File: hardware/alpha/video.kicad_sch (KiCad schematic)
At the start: 104 parts, among them J1 BANK2_AUX, J2 OUT1, J3 OUT2, U1 L78L05_SO8, U3 L79L05_SO8, U4 AD768, U5 MAX4104, U6 AD8620, U7 MAX4104, U8 MCP47FEB22A0-E/ST

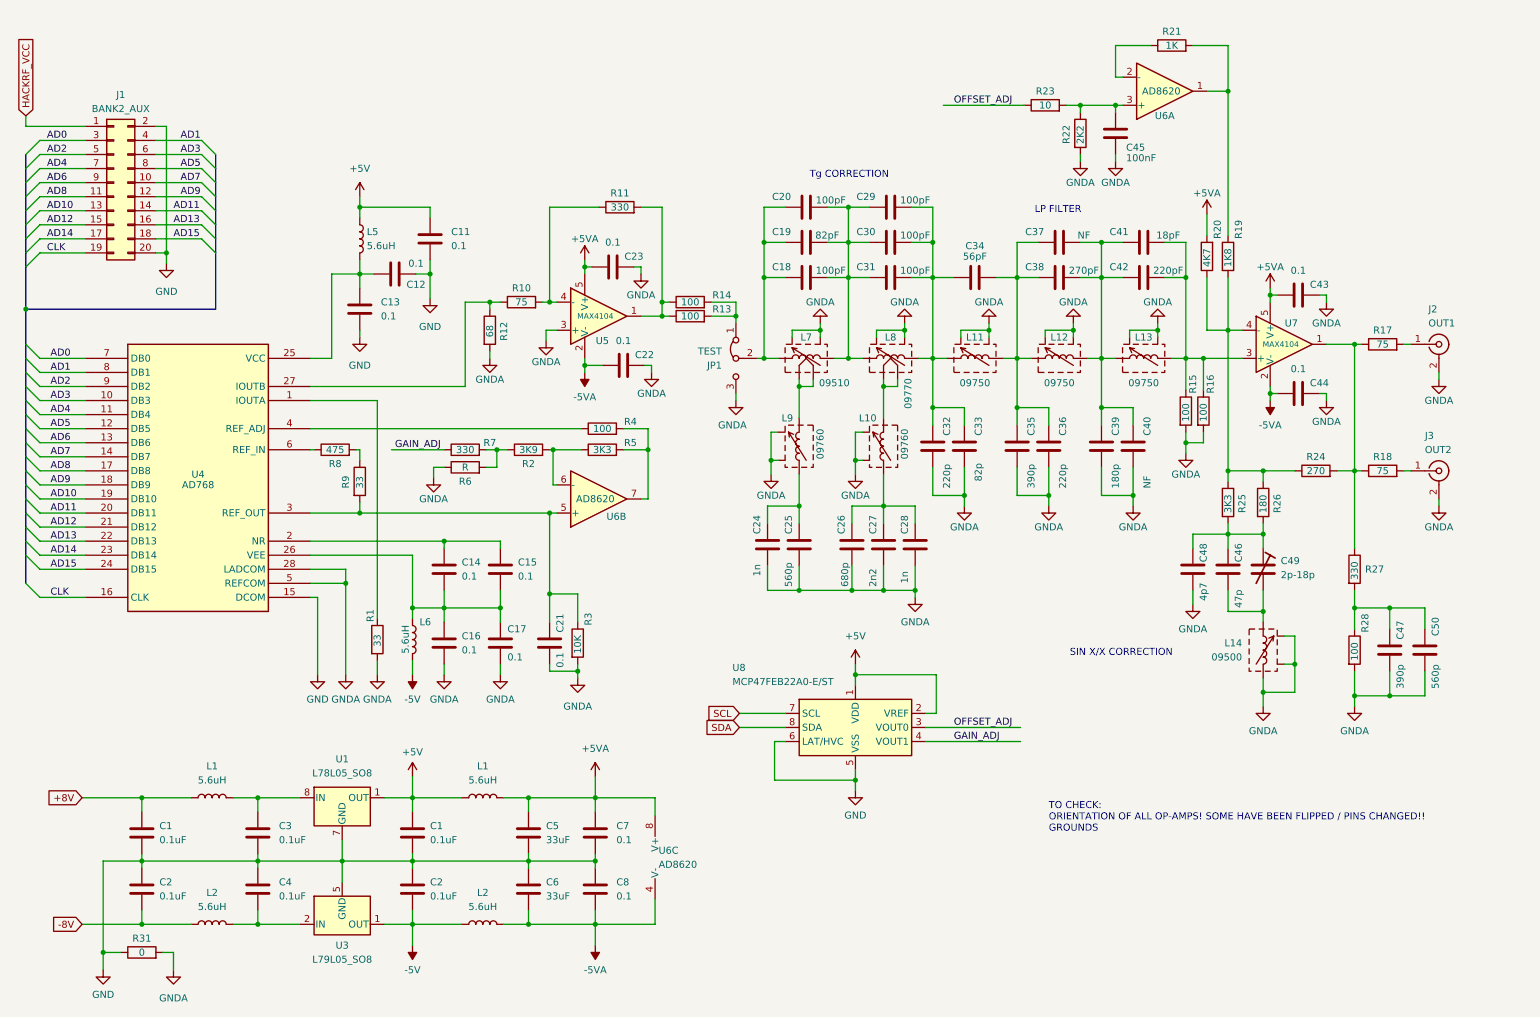
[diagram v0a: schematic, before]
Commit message: Updated
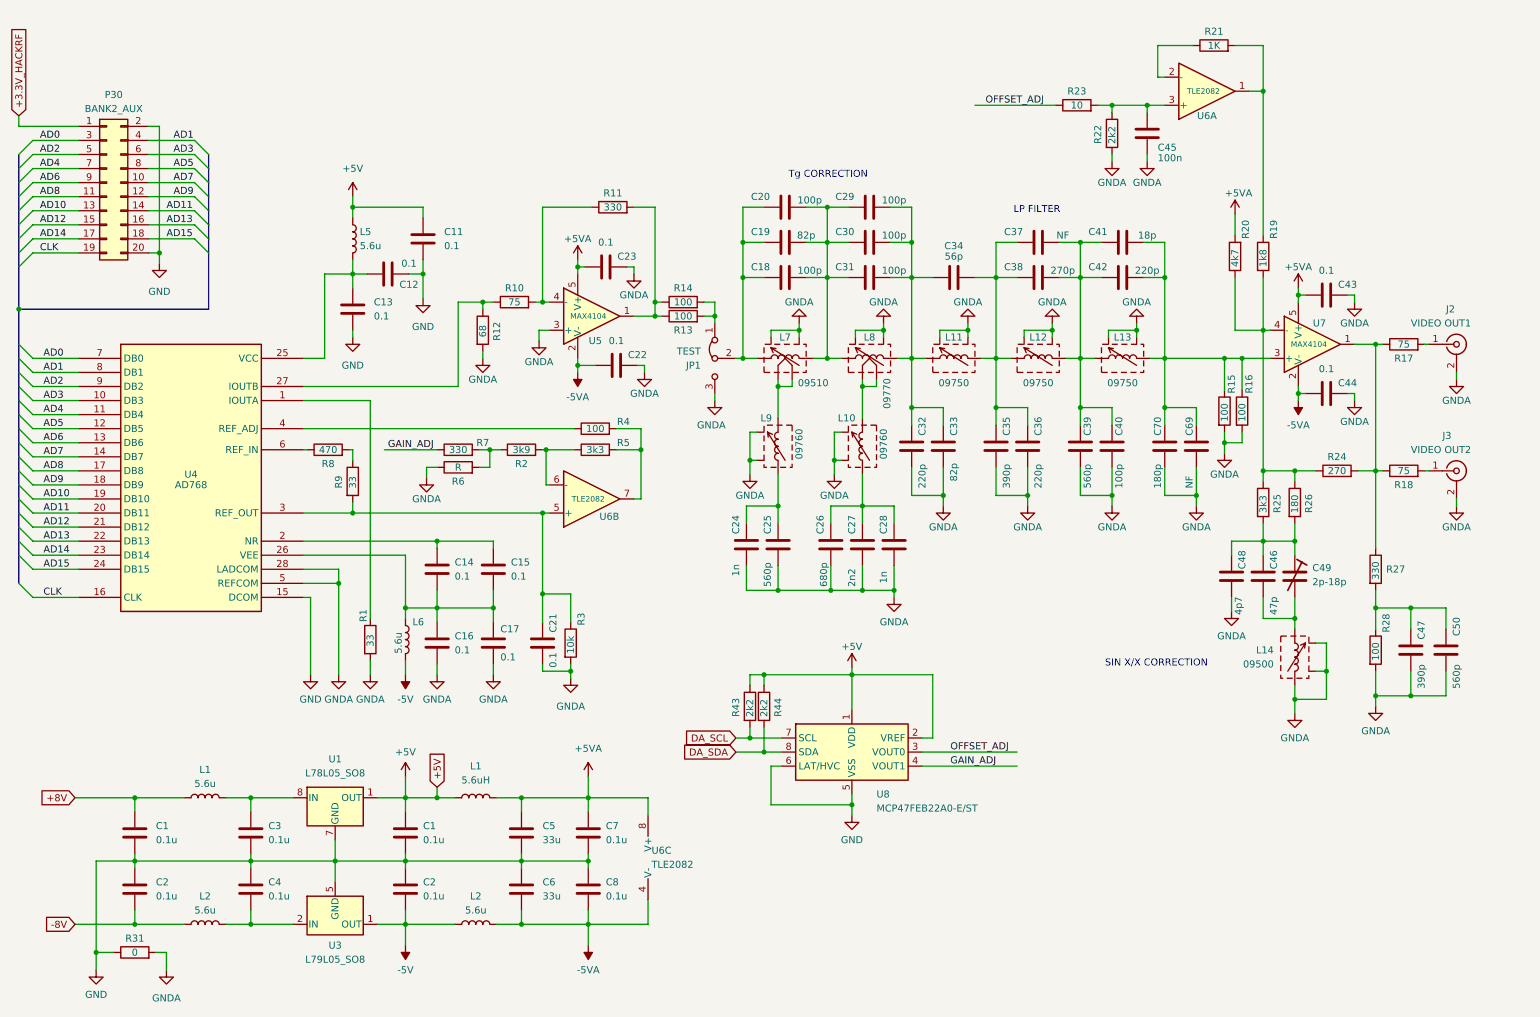
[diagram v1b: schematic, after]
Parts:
- added C69: NF, symbol Device:C
- added C70: 180p, symbol Device:C
- added R43, R44: 2k2, symbol Device:R
- C1, C2, C3, C4: value 0.1uF -> 0.1u
- C18, C20, C29, C30, C31: value 100pF -> 100p
- C19: value 82pF -> 82p
- C34: value 56pF -> 56p
- C38: value 270pF -> 270p
- C39: value 180p -> 560p
- C40: value NF -> 100p
- C41: value 18pF -> 18p
- C42: value 220pF -> 220p
- C45: value 100nF -> 100n
- C5, C6: value 33uF -> 33u
- C7, C8: value 0.1 -> 0.1u
- J2: value OUT1 -> VIDEO OUT1
- J3: value OUT2 -> VIDEO OUT2
- L1, L2, L5, L6: value 5.6uH -> 5.6u
- R19: value 1K8 -> 1k8
- R2: value 3K9 -> 3k9
- R20: value 4K7 -> 4k7
- R22: value 2K2 -> 2k2
- R25, R5: value 3K3 -> 3k3
- R3: value 10K -> 10k
- R8: value 475 -> 470
- U6: value AD8620 -> TLE2082
- renumbered J1 to P30
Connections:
- net +5V: now also R43.1, R44.1
- net GNDA: now also C69.2, C70.2
- net at C41.2, C42.2, L13.4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: now also C69.1, C70.1
- net HACKRF_VCC renamed +3.3V_HACKRF
- net SCL renamed DA_SCL
- net DA_SCL: now also R43.2
- net SDA renamed DA_SDA
- net DA_SDA: now also R44.2
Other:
- note removed: "TO CHECK: ORIENTATION OF ALL OP-AMPS! SOME HAVE BEEN FLIPPED / PINS CHANGED!! GROUNDS"
- moved on the sheet: C1, C11, C12, C13, C14, C15, C16, C17, C18, C19, C2, C20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
